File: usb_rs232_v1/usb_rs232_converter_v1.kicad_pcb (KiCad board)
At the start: 2 copper layers, 59 x 40 mm, 6 parts, among them CON1 USB-MINI-B, CON2 USB-MICRO-B, IC1 MAX3243, J1 DB9, J2 DB9

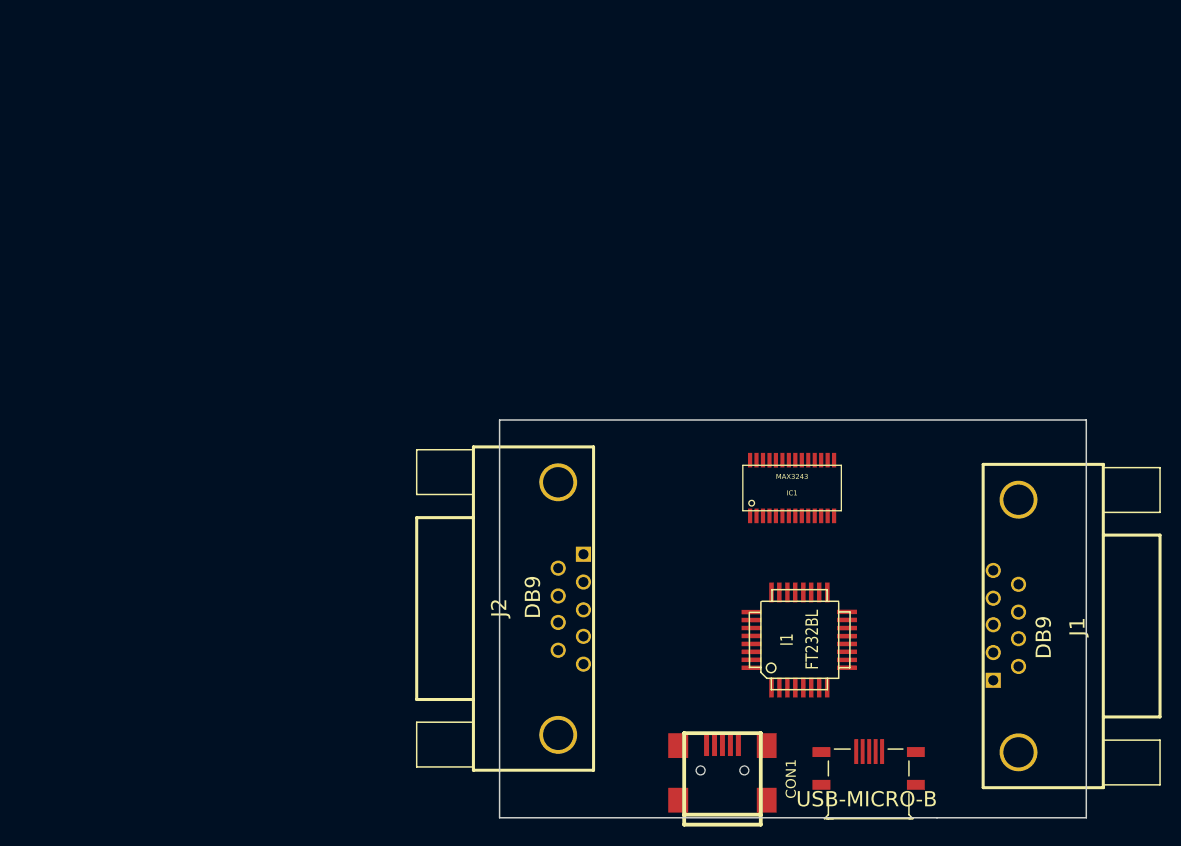
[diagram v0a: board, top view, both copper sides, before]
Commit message: Schemat v1
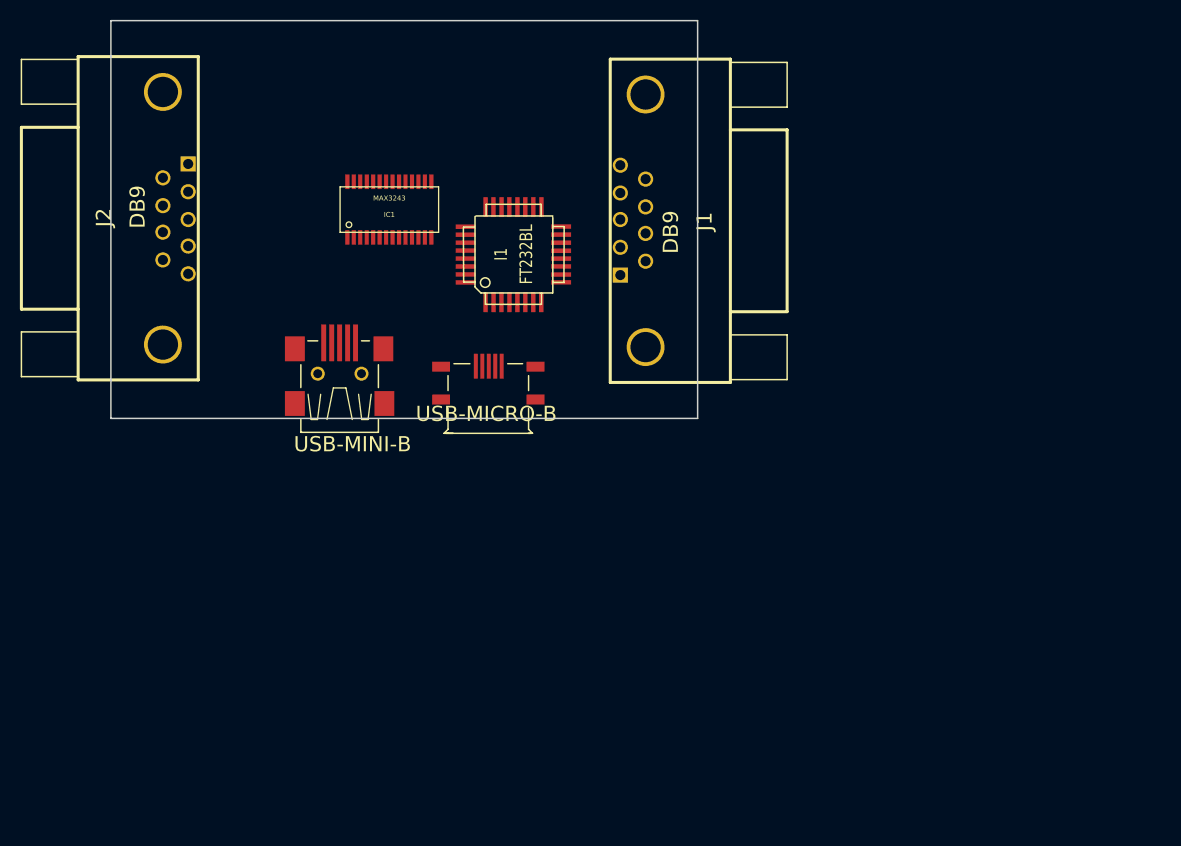
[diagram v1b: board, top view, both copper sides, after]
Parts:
- CON1: footprint USB_MINI_B -> usb-mini-B
- moved CON1 56.1 mm to (59.0, 62.5)
- moved J2 55.9 mm to (42.5, 47.0)
- moved J1 55.4 mm to (88.5, 47.0)
- moved CON2 54.4 mm to (74.0, 65.0)
- moved IC1 49.2 mm to (64.0, 46.0)
- moved I1 48.3 mm to (76.5, 50.5)
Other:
- outline, holes or cut-outs redrawn
- board text removed: "siatki: - 0,508 elementy"
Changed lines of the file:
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@@
     (links 0)
     (no_connects 0)
-    (area 75.009999 67.084999 134.160001 107.235001)
+    (area 65.987999 56.928 146.628859 109.605644)
     (thickness 1.6)
-    (drawings 6)
+    (drawings 4)
     (tracks 0)
     (zones 0)
@@
     (mod_text_size 1 1)
     (mod_text_width 0.15)
-    (pad_size 1 1.8)
+    (pad_size 3.7 0.49784)
     (pad_drill 0)
     (pad_to_mask_clearance 0)
     (aux_axis_origin 0 0)
-    (visible_elements FFFE7501)
+    (visible_elements FFFE7D01)
     (pcbplotparams
       (layerselection 3178497)
@@
   )
   (module TQFP32 (layer F.Cu)
-    (at 105.25 89.25 90)
+    (at 76.5 50.5 90)
     (fp_text reference I1 (at 0 -1.27 90) (layer F.SilkS)
       (effects (font (size 1.27 1.016) (thickness 0.2032)))
@@
     )
   )
-  (module USB_MINI_B (layer F.Cu)
-    (at 97.5 103.25 90)
-    (descr "USB Mini-B 5-pin SMD connector")
-    (tags "USB, Mini-B, connector")
-    (fp_text reference CON1 (at 0 6.90118 90) (layer F.SilkS)
-      (effects (font (size 1.016 1.016) (thickness 0.2032)))
-    )
-    (fp_text value USB-MINI-B (at 0 -7.0993 90) (layer F.SilkS) hide
-      (effects (font (size 1.016 1.016) (thickness 0.2032)))
-    )
-    (fp_line (start -3.59918 -3.85064) (end -3.59918 3.85064) (layer F.SilkS) (width 0.381))
-    (fp_line (start -4.59994 -3.85064) (end -4.59994 3.85064) (layer F.SilkS) (width 0.381))
-    (fp_line (start -4.59994 3.85064) (end 4.59994 3.85064) (layer F.SilkS) (width 0.381))
-    (fp_line (start 4.59994 3.85064) (end 4.59994 -3.85064) (layer F.SilkS) (width 0.381))
-    (fp_line (start 4.59994 -3.85064) (end -4.59994 -3.85064) (layer F.SilkS) (width 0.381))
-    (pad 1 smd rect (at 3.44932 -1.6002 90) (size 2.30124 0.50038)
-      (layers F.Cu F.Paste F.Mask)
-    )
-    (pad 2 smd rect (at 3.44932 -0.8001 90) (size 2.30124 0.50038)
-      (layers F.Cu F.Paste F.Mask)
-    )
-    (pad 3 smd rect (at 3.44932 0 90) (size 2.30124 0.50038)
-      (layers F.Cu F.Paste F.Mask)
-    )
-    (pad 4 smd rect (at 3.44932 0.8001 90) (size 2.30124 0.50038)
-      (layers F.Cu F.Paste F.Mask)
-    )
-    (pad 5 smd rect (at 3.44932 1.6002 90) (size 2.30124 0.50038)
-      (layers F.Cu F.Paste F.Mask)
-    )
-    (pad 6 smd rect (at 3.35026 -4.45008 90) (size 2.49936 1.99898)
-      (layers F.Cu F.Paste F.Mask)
-    )
-    (pad 7 smd rect (at -2.14884 -4.45008 90) (size 2.49936 1.99898)
-      (layers F.Cu F.Paste F.Mask)
-    )
-    (pad 8 smd rect (at 3.35026 4.45008 90) (size 2.49936 1.99898)
-      (layers F.Cu F.Paste F.Mask)
-    )
-    (pad 9 smd rect (at -2.14884 4.45008 90) (size 2.49936 1.99898)
-      (layers F.Cu F.Paste F.Mask)
-    )
-    (pad "" np_thru_hole circle (at 0.8509 -2.19964 90) (size 0.89916 0.89916) (drill 0.89916)
-      (layers *.Cu *.Mask F.SilkS)
-    )
-    (pad 2 np_thru_hole circle (at 0.8509 2.19964 90) (size 0.89916 0.89916) (drill 0.89916)
-      (layers *.Cu *.Mask F.SilkS)
-    )
-  )
   (module tssop-28 (layer F.Cu)
-    (at 104.5 74)
+    (at 64 46)
     (descr TSSOP-28)
     (fp_text reference IC1 (at 0 0.508) (layer F.SilkS)
@@
   )
   (module usb-micro-B (layer F.Cu)
-    (at 112.25 103.75 90)
+    (at 74 65 90)
     (descr "USB SERIES MINI-B SURFACE MOUNTED")
     (tags "USB SERIES MINI-B SURFACE MOUNTED")
@@
   )
   (module DB9MC-v2 (layer F.Cu)
-    (at 126 87.75 270)
+    (at 88.5 47 270)
     (descr "Connecteur DB9 male couche")
     (tags "CONN DB9")
@@
   )
   (module DB9MC-v2 (layer F.Cu)
-    (at 82.25 86.25 90)
+    (at 42.5 47 90)
     (descr "Connecteur DB9 male couche")
     (tags "CONN DB9")
@@
     )
   )
-  (gr_line (start 75.085 67.16) (end 75.085 107.16) (angle 90) (layer Edge.Cuts) (width 0.15))
-  (gr_line (start 134.085 67.16) (end 75.085 67.16) (angle 90) (layer Edge.Cuts) (width 0.15))
-  (gr_line (start 134.085 107.16) (end 134.085 67.16) (angle 90) (layer Edge.Cuts) (width 0.15))
-  (gr_line (start 119.085 107.16) (end 134.085 107.16) (angle 90) (layer Edge.Cuts) (width 0.15))
-  (gr_line (start 75.085 107.16) (end 119.085 107.16) (angle 90) (layer Edge.Cuts) (width 0.15))
-  (gr_text "siatki:\n- 0,508 elementy\n\n" (at 105.336 59.478) (layer Cmts.User)
-    (effects (font (size 3 3) (thickness 0.3)) (justify left))
-  )
+  (module usb-mini-B (layer F.Cu)
+    (at 59 62.5 90)
+    (descr "USB SERIES MINI-B SURFACE MOUNTED")
+    (tags "USB SERIES MINI-B SURFACE MOUNTED")
+    (attr smd)
+    (fp_text reference CON1 (at 6.1 -5.1 180) (layer B.SilkS)
+      (effects (font (size 1.27 1.27) (thickness 0.0889)))
+    )
+    (fp_text value USB-MINI-B (at -7.1 1.3 180) (layer F.SilkS)
+      (effects (font (size 1.524 1.524) (thickness 0.15)))
+    )
+    (fp_line (start -1.4 -3.9) (end 0.9 -3.9) (layer F.SilkS) (width 0.15))
+    (fp_line (start -5.9 -3.8) (end -5.9 -3.9) (layer F.SilkS) (width 0.15))
+    (fp_line (start -5.9 -3.9) (end -4.6 -3.9) (layer F.SilkS) (width 0.15))
+    (fp_line (start -5.9 3.9) (end -5.9 -3.8) (layer F.SilkS) (width 0.15))
+    (fp_line (start -1.4 3.9) (end 0.9 3.9) (layer F.SilkS) (width 0.15))
+    (fp_line (start -5.9 3.9) (end -4.6 3.9) (layer F.SilkS) (width 0.15))
+    (fp_line (start 3.3 3) (end 3.3 2.2) (layer F.SilkS) (width 0.15))
+    (fp_line (start 3.3 -3.2) (end 3.3 -2.2) (layer F.SilkS) (width 0.15))
+    (fp_line (start -4.61264 -1.27) (end -1.43764 -0.635) (layer F.SilkS) (width 0.127))
+    (fp_line (start -1.43764 -0.635) (end -1.43764 0.635) (layer F.SilkS) (width 0.127))
+    (fp_line (start -1.43764 0.635) (end -4.61264 1.27) (layer F.SilkS) (width 0.127))
+    (fp_line (start -2.07264 3.175) (end -4.61264 2.8575) (layer F.SilkS) (width 0.127))
+    (fp_line (start -4.61264 2.8575) (end -4.61264 2.2225) (layer F.SilkS) (width 0.127))
+    (fp_line (start -4.61264 2.2225) (end -2.07264 1.905) (layer F.SilkS) (width 0.127))
+    (fp_line (start -2.07264 -3.175) (end -4.61264 -2.8575) (layer F.SilkS) (width 0.127))
+    (fp_line (start -4.61264 -2.8575) (end -4.61264 -2.2225) (layer F.SilkS) (width 0.127))
+    (fp_line (start -4.61264 -2.2225) (end -2.07264 -1.905) (layer F.SilkS) (width 0.127))
+    (pad D+ smd rect (at 3.1 0 90) (size 3.7 0.49784)
+      (layers F.Cu F.Paste F.Mask)
+    )
+    (pad D- smd rect (at 3.1 -0.8 90) (size 3.7 0.49784)
+      (layers F.Cu F.Paste F.Mask)
+    )
+    (pad GND smd rect (at 3.1 1.6 90) (size 3.7 0.49784)
+      (layers F.Cu F.Paste F.Mask)
+    )
+    (pad ID smd rect (at 3.1 0.8 90) (size 3.7 0.49784)
+      (layers F.Cu F.Paste F.Mask)
+    )
+    (pad P$1 smd rect (at -2.99974 4.49834 90) (size 2.49936 1.99898)
+      (layers F.Cu F.Paste F.Mask)
+    )
+    (pad P$2 smd rect (at -2.99974 -4.49834 90) (size 2.49936 1.99898)
+      (layers F.Cu F.Paste F.Mask)
+    )
+    (pad P$3 smd rect (at 2.49936 4.39928 90) (size 2.49936 1.99898)
+      (layers F.Cu F.Paste F.Mask)
+    )
+    (pad P$4 smd rect (at 2.49936 -4.49834 90) (size 2.49936 1.99898)
+      (layers F.Cu F.Paste F.Mask)
+    )
+    (pad P$5 thru_hole circle (at 0 -2.19964 90) (size 1.40716 1.40716) (drill 0.89916)
+      (layers *.Cu F.Paste F.SilkS F.Mask)
+    )
+    (pad P$6 thru_hole circle (at 0 2.19964 90) (size 1.40716 1.40716) (drill 0.89916)
+      (layers *.Cu F.Paste F.SilkS F.Mask)
+    )
+    (pad VCC smd rect (at 3.1 -1.6 90) (size 3.7 0.49784)
+      (layers F.Cu F.Paste F.Mask)
+    )
+  )
+  (gr_line (start 36 67) (end 36 27) (angle 90) (layer Edge.Cuts) (width 0.15))
+  (gr_line (start 95 67) (end 36 67) (angle 90) (layer Edge.Cuts) (width 0.15))
+  (gr_line (start 95 27) (end 95 67) (angle 90) (layer Edge.Cuts) (width 0.15))
+  (gr_line (start 36 27) (end 95 27) (angle 90) (layer Edge.Cuts) (width 0.15))
 )
